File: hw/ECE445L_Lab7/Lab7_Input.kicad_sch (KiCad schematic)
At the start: 22 parts, among them SW2 Pause, SW3 LCDMode, SW4 Flanger, SW5 Distortion, SW6 Reverb, SW7 Delay, SW8 Tempo

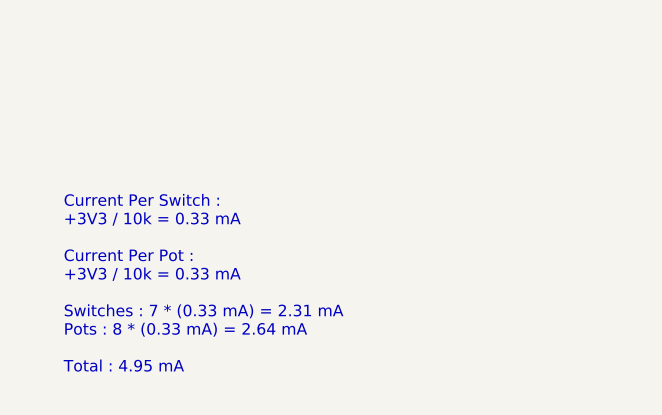
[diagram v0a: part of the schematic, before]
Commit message: Updated lab7a report
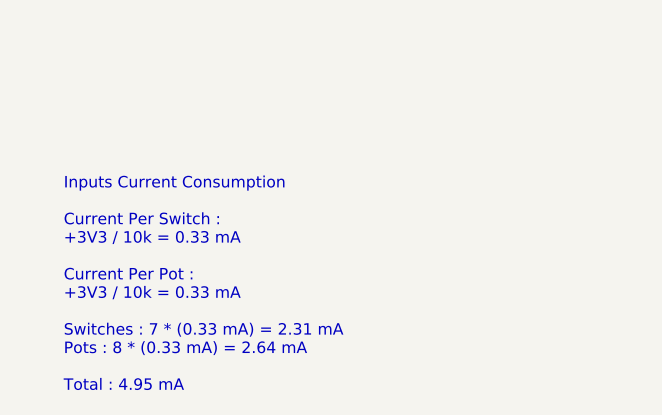
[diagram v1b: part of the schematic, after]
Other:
- note added: "Inputs Current Consumption Current Per Switch : +3V3 / 10k = 0.33 mA Current Per Pot : +3V3 / 10k = 0.33 mA Switches : 7 * (0.33 mA) = 2.31 mA Pots : 8 * (0.33 mA) = 2.64 mA Total : 4.95 mA"
- note removed: "Current Per Switch : +3V3 / 10k = 0.33 mA Current Per Pot : +3V3 / 10k = 0.33 mA Switches : 7 * (0.33 mA) = 2.31 mA Pots : 8 * (0.33 mA) = 2.64 mA Total : 4.95 mA"
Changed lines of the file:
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@@
 		(comment 1 "Drawn By Ashton Knecht - atk836")
 	)
-	(text "Current Per Switch :\n+3V3 / 10k = 0.33 mA\n\nCurrent Per Pot :\n+3V3 / 10k = 0.33 mA\n\nSwitches : 7 * (0.33 mA) = 2.31 mA\nPots : 8 * (0.33 mA) = 2.64 mA\n\nTotal : 4.95 mA"
+	(text "Inputs Current Consumption\n\nCurrent Per Switch :\n+3V3 / 10k = 0.33 mA\n\nCurrent Per Pot :\n+3V3 / 10k = 0.33 mA\n\nSwitches : 7 * (0.33 mA) = 2.31 mA\nPots : 8 * (0.33 mA) = 2.64 mA\n\nTotal : 4.95 mA"
 		(exclude_from_sim no)
 		(at 36.195 182.88 0)
